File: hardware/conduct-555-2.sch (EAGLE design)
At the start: 9 parts, among them J2 AYZ0202

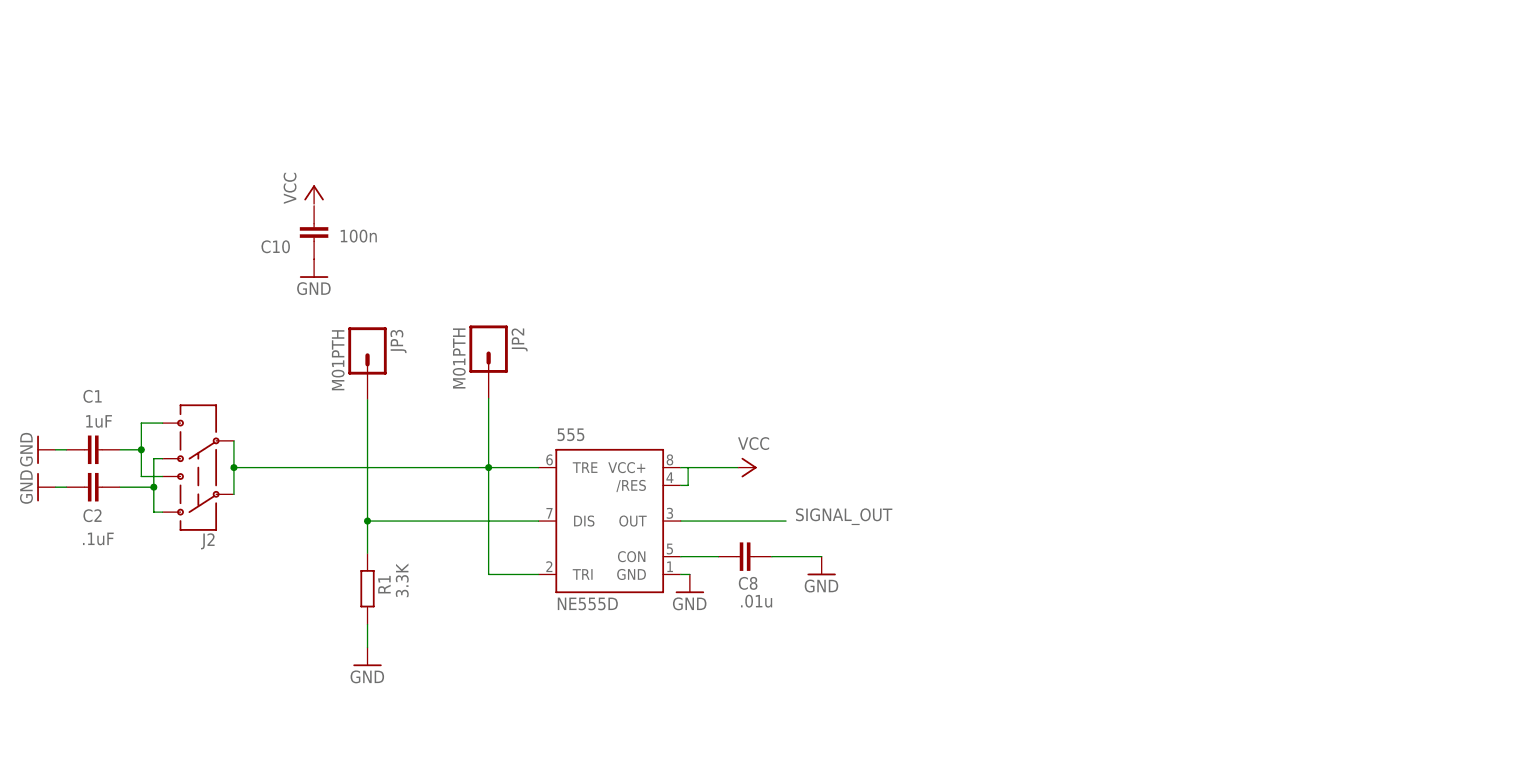
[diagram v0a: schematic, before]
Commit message: update
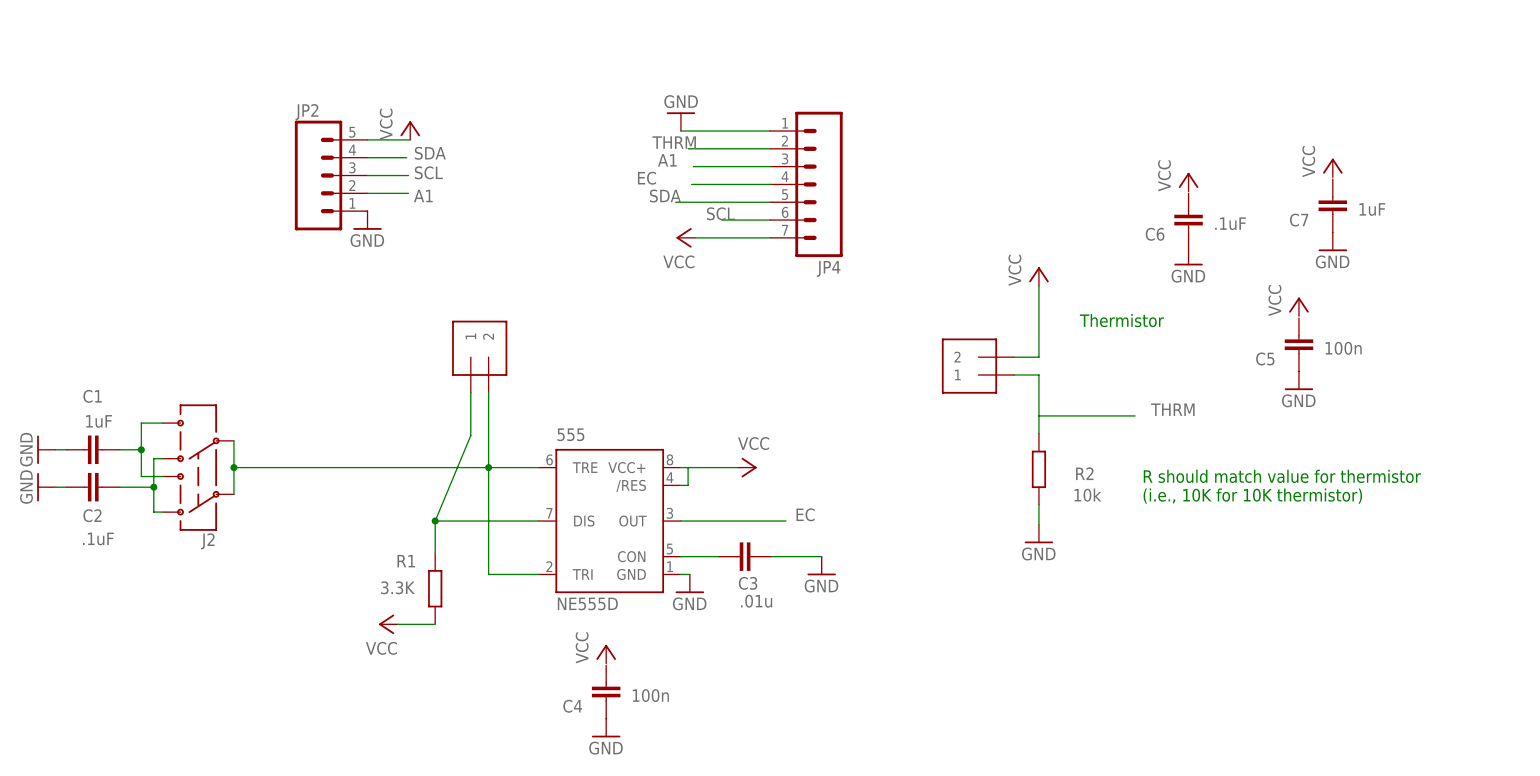
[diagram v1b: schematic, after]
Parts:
- removed C10: 100n, resistor:C-EUC0805
- removed JP3: M01PTH, SparkFun-Connectors:M01PTH
- added C4, C5: 100n, resistor:C-EUC0805
- added C6: .1uF, resistor:C-EUC0805
- added C7: 1uF, resistor:C-EUC0805
- added J-EC, J-THRM: 1X2-3.5MM, adafruit:1X2-3.5MM
- added JP4: (no value), SparkFun-Connectors:M07
- added R2: 10k, rcl:R-EU_R0805
- JP2: value M01PTH -> (none); device SparkFun-Connectors:M01PTH -> SparkFun-Connectors:M05PTH
- renumbered C8 to C3
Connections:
- removed net SIGNAL_OUT: 555.OUT
- new net A1: JP2.2, JP4.3
- new net EC: 555.OUT, JP4.4
- new net SCL: JP2.3, JP4.6
- new net SDA: JP2.4, JP4.5
- new net THRM: J-THRM.1, JP4.2, R2.2
- net GND: now also C4.1, C5.1, C6.1, C7.1, JP2.1, JP4.1, R2.1; no longer C10.1, R1.1
- net N$3: now also J-EC.1; no longer JP3.1
- net N1: now also J-EC.2; no longer JP2.1
- net VCC: now also J-THRM.2, JP2.5, JP4.7, R1.1
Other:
- note added: "R should match value for thermistor (i.e., 10K for 10K thermistor)"
- note added: "Thermistor"
- moved on the sheet: R1

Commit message: update
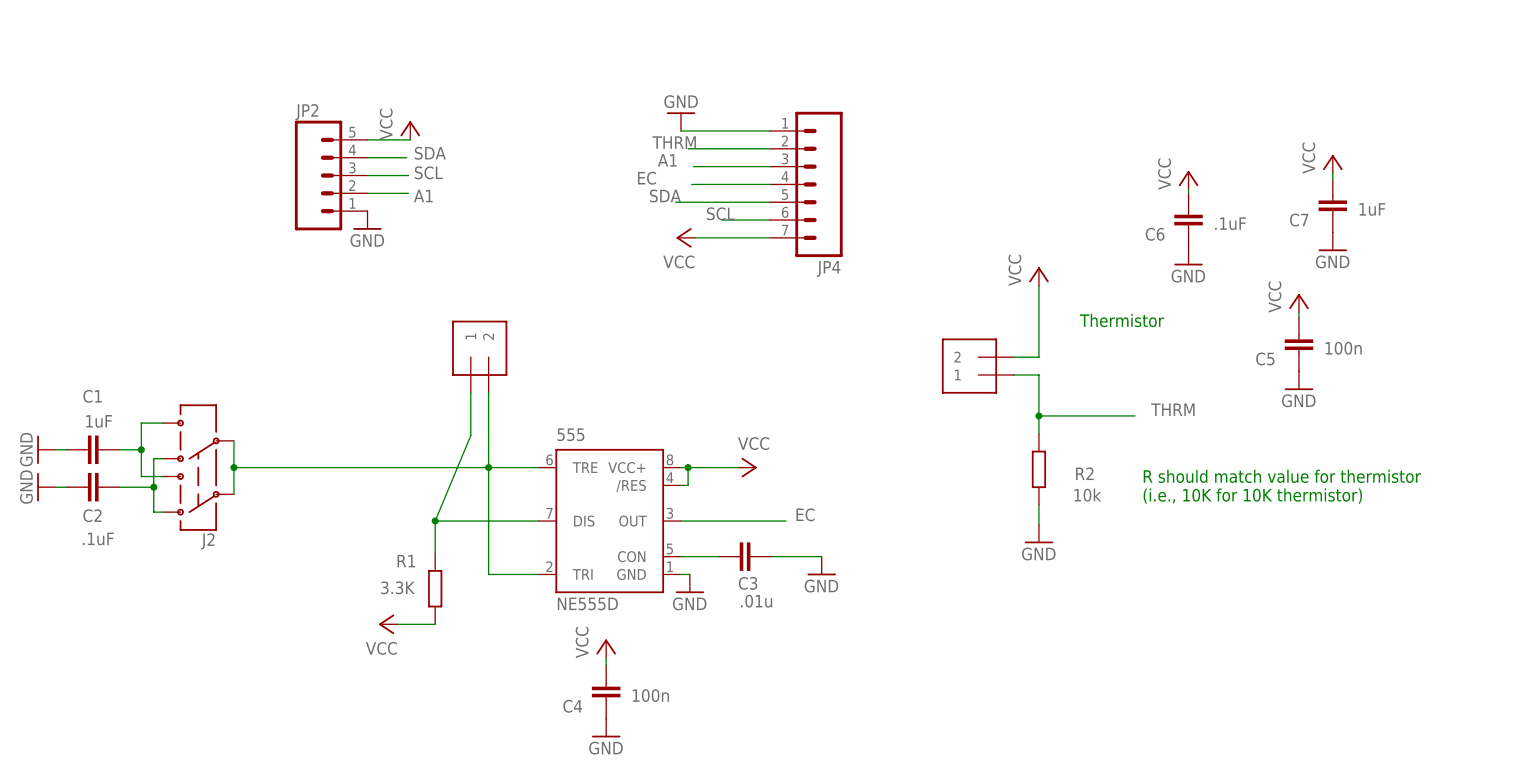
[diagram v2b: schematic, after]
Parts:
- renumbered J-EC to EC, J-THRM to THRM
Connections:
- net VCC: now also C4.2, C5.2, C6.2, C7.2
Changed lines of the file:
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@@
 <setting verticaltext="up"/>
 </settings>
-<grid distance="0.01" unitdist="inch" unit="inch" style="lines" multiple="1" display="no" altdistance="0.01" altunitdist="inch" altunit="inch"/>
+<grid distance="0.1" unitdist="inch" unit="inch" style="lines" multiple="1" display="no" altdistance="0.01" altunitdist="inch" altunit="inch"/>
 <layers>
 <layer number="1" name="Top" color="4" fill="1" visible="no" active="no"/>
@@
 <part name="GND1" library="SparkFun" deviceset="GND" device=""/>
 <part name="R1" library="rcl" deviceset="R-EU_" device="R0805" value="3.3K"/>
-<part name="J-THRM" library="adafruit" deviceset="1X2" device="-3.5MM"/>
+<part name="THRM" library="adafruit" deviceset="1X2" device="-3.5MM"/>
 <part name="P+3" library="supply1" deviceset="VCC" device=""/>
 <part name="P+5" library="supply1" deviceset="VCC" device=""/>
@@
 <part name="GND2" library="SparkFun" deviceset="GND" device=""/>
 <part name="JP4" library="SparkFun-Connectors" deviceset="M07" device=""/>
-<part name="J-EC" library="adafruit" deviceset="1X2" device="-3.5MM"/>
+<part name="EC" library="adafruit" deviceset="1X2" device="-3.5MM"/>
 <part name="P+1" library="supply1" deviceset="VCC" device=""/>
 <part name="C5" library="resistor" deviceset="C-EU" device="C0805" value="100n"/>
@@
 </instance>
 <instance part="GND9" gate="1" x="98.298" y="26.67"/>
-<instance part="P+4" gate="VCC" x="98.298" y="39.624"/>
+<instance part="P+4" gate="VCC" x="98.298" y="40.386"/>
 <instance part="555" gate="G$1" x="98.806" y="57.404"/>
 <instance part="J2" gate="G$1" x="40.132" y="63.754" smashed="yes" rot="R180">
@@
 <attribute name="VALUE" x="66.04" y="46.99" size="1.778" layer="96"/>
 </instance>
-<instance part="J-THRM" gate="G$1" x="151.384" y="80.772" rot="R180"/>
+<instance part="THRM" gate="G$1" x="151.384" y="80.772" rot="R180"/>
 <instance part="P+3" gate="VCC" x="66.04" y="42.672" rot="R90"/>
 <instance part="P+5" gate="VCC" x="160.02" y="93.472"/>
@@
 <instance part="GND2" gate="1" x="160.02" y="54.356"/>
 <instance part="JP4" gate="G$1" x="126.746" y="107.95" rot="R180"/>
-<instance part="J-EC" gate="G$1" x="81.534" y="80.772" rot="R90"/>
+<instance part="EC" gate="G$1" x="81.534" y="80.772" rot="R90"/>
 <instance part="P+1" gate="VCC" x="108.458" y="97.79" rot="R90"/>
 <instance part="C5" gate="G$1" x="197.104" y="81.28" smashed="yes" rot="R180">
@@
 </instance>
 <instance part="GND3" gate="1" x="197.104" y="76.2"/>
-<instance part="P+6" gate="VCC" x="197.104" y="89.154"/>
+<instance part="P+6" gate="VCC" x="197.104" y="89.662"/>
 <instance part="C6" gate="G$1" x="181.356" y="99.06" smashed="yes" rot="R180">
 <attribute name="NAME" x="178.054" y="99.187" size="1.778" layer="95" rot="R180"/>
@@
 </instance>
 <instance part="GND5" gate="1" x="181.356" y="93.98"/>
-<instance part="P+7" gate="VCC" x="181.356" y="106.934"/>
+<instance part="P+7" gate="VCC" x="181.356" y="107.188"/>
 <instance part="C7" gate="G$1" x="201.93" y="101.092" smashed="yes" rot="R180">
 <attribute name="NAME" x="198.628" y="101.219" size="1.778" layer="95" rot="R180"/>
@@
 </instance>
 <instance part="GND6" gate="1" x="201.93" y="96.012"/>
-<instance part="P+8" gate="VCC" x="201.93" y="108.966"/>
+<instance part="P+8" gate="VCC" x="201.93" y="109.474"/>
 <instance part="GND7" gate="1" x="108.966" y="115.57" rot="R180"/>
 <instance part="GND8" gate="1" x="64.262" y="99.06"/>
@@
 <wire x1="81.534" y1="65.024" x2="81.534" y2="75.692" width="0.1524" layer="91"/>
 <junction x="81.534" y="65.024"/>
-<pinref part="J-EC" gate="G$1" pin="2"/>
+<pinref part="EC" gate="G$1" pin="2"/>
 </segment>
 </net>
@@
 <wire x1="109.982" y1="65.024" x2="117.094" y2="65.024" width="0.1524" layer="91"/>
 <pinref part="P+2" gate="VCC" pin="VCC"/>
+<junction x="109.982" y="65.024"/>
 </segment>
 <segment>
@@
 <segment>
 <pinref part="P+5" gate="VCC" pin="VCC"/>
-<pinref part="J-THRM" gate="G$1" pin="2"/>
+<pinref part="THRM" gate="G$1" pin="2"/>
 <wire x1="156.464" y1="80.772" x2="160.02" y2="80.772" width="0.1524" layer="91"/>
 <wire x1="160.02" y1="80.772" x2="160.02" y2="90.932" width="0.1524" layer="91"/>
@@
 <wire x1="70.358" y1="111.76" x2="64.262" y2="111.76" width="0.1524" layer="91"/>
 <pinref part="JP2" gate="G$1" pin="5"/>
+</segment>
+<segment>
+<pinref part="C4" gate="G$1" pin="2"/>
+<pinref part="P+4" gate="VCC" pin="VCC"/>
+<wire x1="98.298" y1="37.846" x2="98.298" y2="36.83" width="0.1524" layer="91"/>
+</segment>
+<segment>
+<pinref part="C5" gate="G$1" pin="2"/>
+<pinref part="P+6" gate="VCC" pin="VCC"/>
+<wire x1="197.104" y1="87.122" x2="197.104" y2="86.36" width="0.1524" layer="91"/>
+</segment>
+<segment>
+<pinref part="C6" gate="G$1" pin="2"/>
+<pinref part="P+7" gate="VCC" pin="VCC"/>
+<wire x1="181.356" y1="104.648" x2="181.356" y2="104.14" width="0.1524" layer="91"/>
+</segment>
+<segment>
+<pinref part="C7" gate="G$1" pin="2"/>
+<pinref part="P+8" gate="VCC" pin="VCC"/>
+<wire x1="201.93" y1="106.934" x2="201.93" y2="106.172" width="0.1524" layer="91"/>
 </segment>
 </net>
@@
 <wire x1="78.994" y1="69.596" x2="73.914" y2="57.404" width="0.1524" layer="91"/>
 <junction x="73.914" y="57.404"/>
-<pinref part="J-EC" gate="G$1" pin="1"/>
+<pinref part="EC" gate="G$1" pin="1"/>
 <wire x1="78.994" y1="75.692" x2="78.994" y2="69.596" width="0.1524" layer="91"/>
 </segment>
@@
 <net name="THRM" class="0">
 <segment>
-<pinref part="J-THRM" gate="G$1" pin="1"/>
+<pinref part="THRM" gate="G$1" pin="1"/>
 <wire x1="156.464" y1="78.232" x2="160.02" y2="78.232" width="0.1524" layer="91"/>
 <wire x1="160.02" y1="78.232" x2="160.02" y2="72.39" width="0.1524" layer="91"/>
@@
 <wire x1="160.02" y1="72.39" x2="173.736" y2="72.39" width="0.1524" layer="91"/>
 <label x="176.022" y="72.39" size="1.778" layer="95"/>
-</segment>
-<segment>
+<junction x="160.02" y="72.39"/>
+</segment>
+<segment>
